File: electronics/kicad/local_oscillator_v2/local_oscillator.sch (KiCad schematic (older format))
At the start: 17 parts, among them P1 TestPoint:TestPoint_Pad_1.5x1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, P3 TestPoint:TestPoint_Pad_1.5x1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, P4 TestPoint:TestPoint_Pad_1.5x1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, U1 CE3520K3

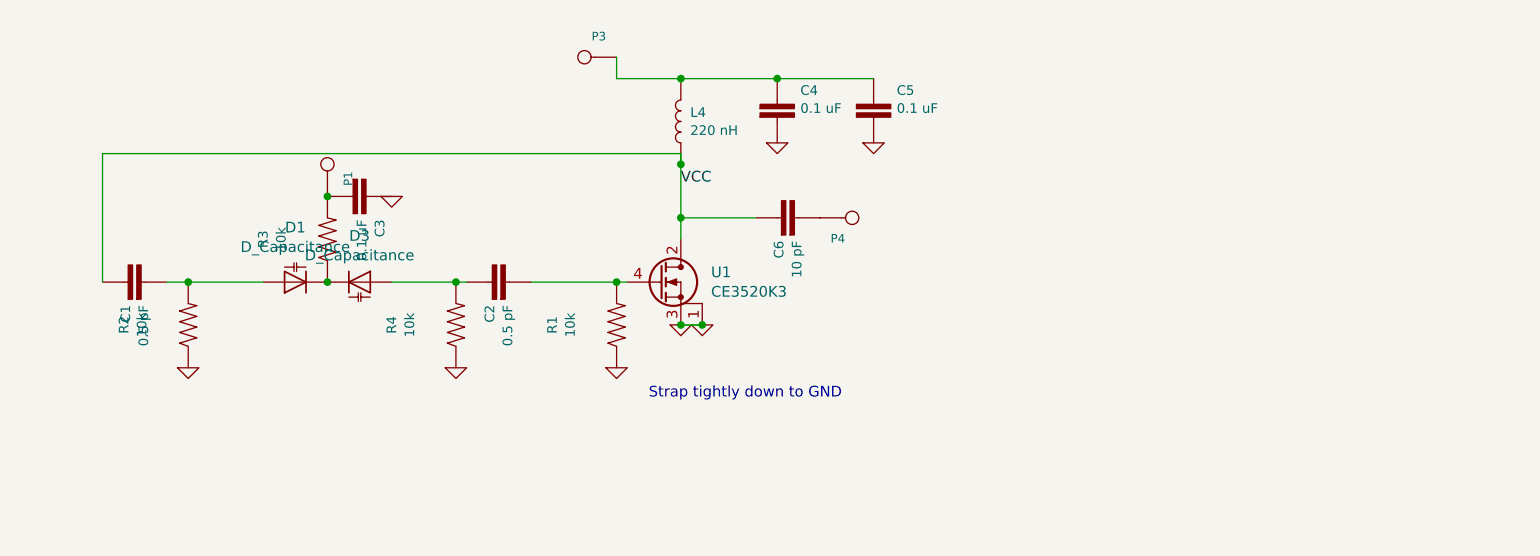
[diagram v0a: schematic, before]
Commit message: Paper
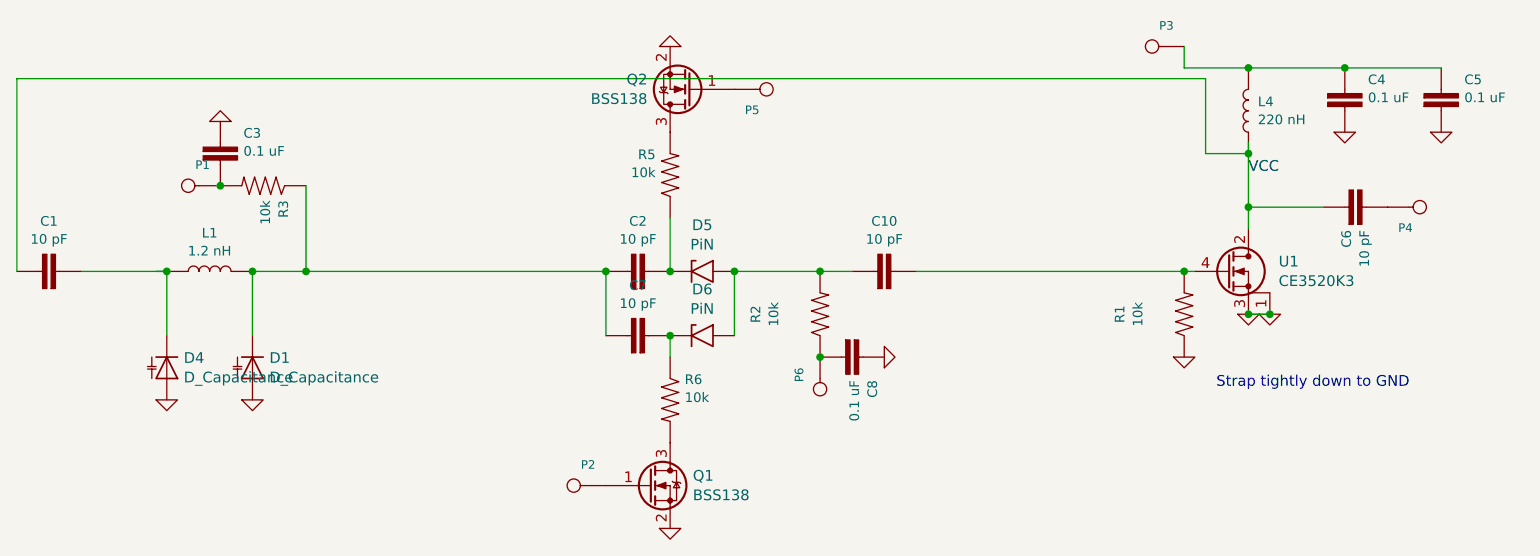
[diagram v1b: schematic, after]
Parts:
- removed D3: D_Capacitance, Diode_SMD:D_SOD-523, symbol Device:D_Capacitance
- removed R4: 10k, 0402, symbol SparkFun-Resistors:RESISTOR0402
- added C10, C7: 10 pF, 0402, symbol SparkFun-Capacitors:6PF-0402-50V-0.5%
- added C8: 0.1 uF, 0603, symbol SparkFun-Capacitors:4.7UF0603
- added D4: D_Capacitance, Diode_SMD:D_SOD-523, symbol Device:D_Capacitance
- added D5, D6: PiN, Diode_SMD:D_SOD-523, symbol Diode:1.5KExxA
- added L1: 1.2 nH, 0402, symbol SparkFun-Coils:INDUCTOR-0402-3.9NH
- added P2, P5, P6: TestPoint:TestPoint_Pad_1.5x1.5mm, TestPoint:TestPoint_Pad_1.5x1.5mm, symbol conn:CONN_1
- added Q1, Q2: BSS138, Package_TO_SOT_SMD:SOT-23, symbol Transistor_FET:BSS138
- added R5, R6: 10k, 0402, symbol SparkFun-Resistors:RESISTOR0402
- C1, C2: value 0.5 pF -> 10 pF
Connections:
- wire segments 17 -> 28
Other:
- moved on the sheet: C1, C3, C4, C5, C6, D1, L4, P1, P3, P4, R1, R3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
